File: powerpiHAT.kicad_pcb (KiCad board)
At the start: 2 copper layers, 65 x 30 mm, 36 parts, among them J1 Conn_01x10, J2 AudioJack2_Dual_Ground_Switche, J3 40HAT, J4 AudioJack2_Dual_Ground_Switche, J5 AudioJack2_Dual_Ground_Switche, J6 AudioJack2_Dual_Ground_Switche, J9 CONN_01X02, Q1 DMG2305UX, Q2 DMMT5401, U2 CAT24C32

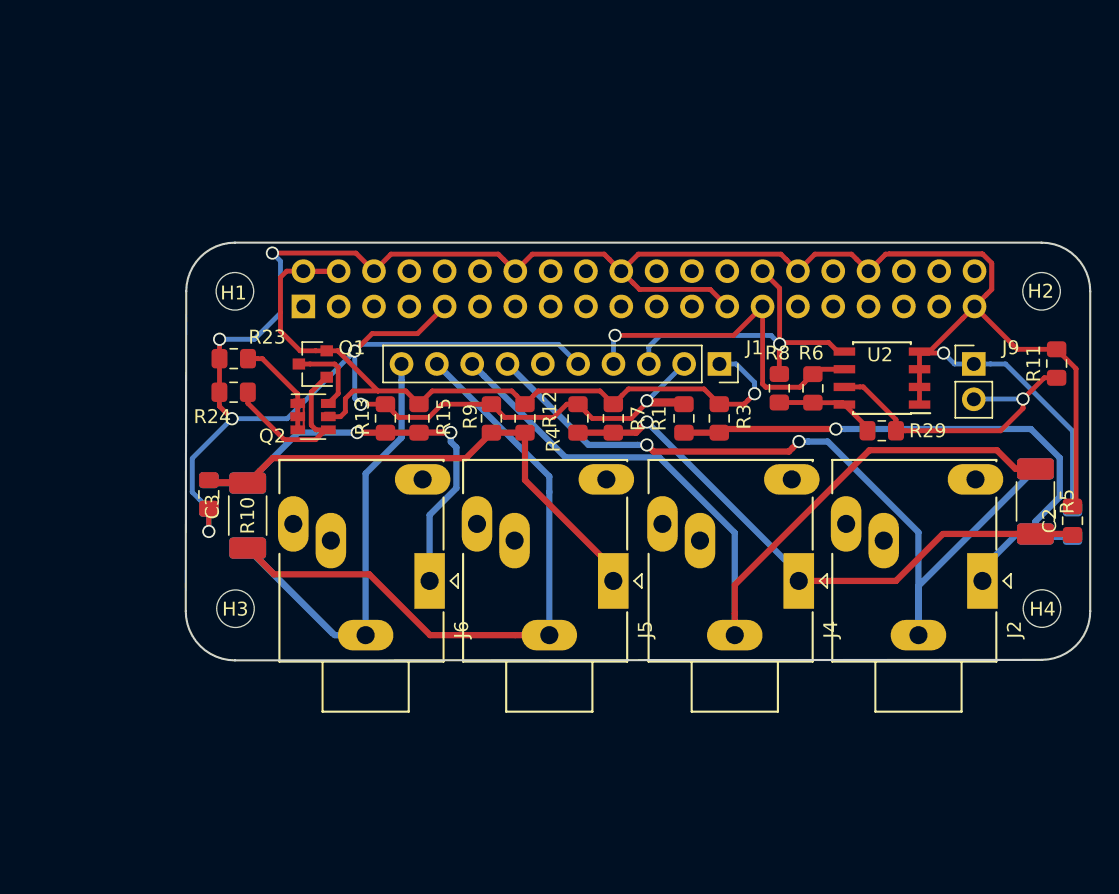
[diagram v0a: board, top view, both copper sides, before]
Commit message: Essentially, release 1.0.0 of the PowerPiHAT... we'll see if there's electrical changes necessary once we get a couple boards etched and populated.
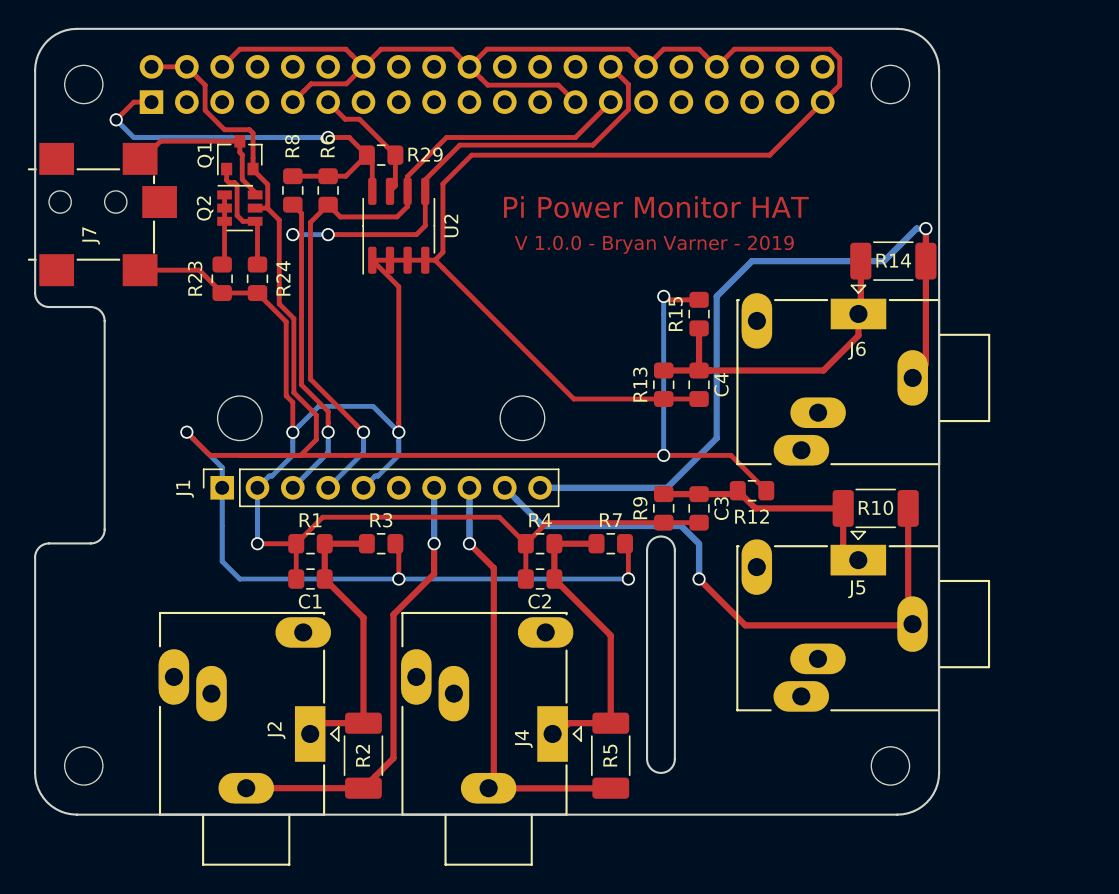
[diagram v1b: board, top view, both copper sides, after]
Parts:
- removed J9: CONN_01X02, Connector_PinHeader_2.54mm:PinHeader_1x02_P2.54mm_Vertical
- removed R11: DNP, Resistor_SMD:R_0805_2012Metric_Pad1.15x1.40mm_HandSolder
- added H5: 3mm_Mounting_Hole, MountingHole:MountingHole_3.2mm_M3_DIN965, F.Cu at (112.7, 88.0)
- added H6: 3mm_Mounting_Hole, MountingHole:MountingHole_3.2mm_M3_DIN965, F.Cu at (133.0, 88.0)
- added J7: Barrel_Jack, project_footprints:BarrellJack-DC-902_SMT_Horizontal, F.Cu at (97.3, 70.3)
- C1, C4, R14, R2: moved to F.Cu
- U2: footprint Package_SOIC:SOIC-8_3.9x4.9mm_P1.27mm -> Package_SO:SOIC-8_3.9x4.9mm_P1.27mm
- moved H4 69.8 mm to (101.5, 113.0)
- moved C1 54.9 mm to (117.8, 99.6), turned to 180 degrees
- moved R2 51.7 mm to (121.6, 112.3), turned to 90 degrees
- moved R14 49.9 mm to (159.7, 76.7), turned to 180 degrees
- moved J2 49.6 mm to (117.8, 110.7)
- moved H3 48.4 mm to (159.5, 113.0)
- moved R10 45.2 mm to (158.4, 94.5), turned to 180 degrees
- moved R29 41.1 mm to (122.9, 69.1)
- moved C2 38.5 mm to (134.3, 99.6), turned to 180 degrees
- moved R8 37.8 mm to (116.5, 71.6), turned to 270 degrees
- moved R6 37.6 mm to (119.1, 71.6), turned to 270 degrees
- moved J1 36.8 mm to (111.5, 93.0), turned to 90 degrees
- moved U2 36.4 mm to (124.2, 74.2), turned to 90 degrees
- moved J6 36.3 mm to (157.2, 80.5), turned to 180 degrees
- moved C4 36.1 mm to (145.7, 85.6)
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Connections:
- J3 pad 1: (no net) -> /P3V3_HAT
- J3 pad 11: (no net) -> /WP_EEPROM
- R29 pad 1: /P3V3 -> /P3V3_HAT
- R29 pad 2: Net-(J9-Pad2) -> /WP_EEPROM
- R6 pad 1: /P3V3 -> /P3V3_HAT
- R8 pad 1: /P3V3 -> /P3V3_HAT
- U2 pad 7: Net-(J9-Pad2) -> /WP_EEPROM
- U2 pad 8: /P3V3 -> /P3V3_HAT
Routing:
- net /P5V_HAT: track 59.3 -> 144.0 mm, vias 1 -> 5
- net /ID_SC_EEPROM: track 24.1 -> 55.9 mm, vias 1 -> 3
- net /P3V3_HAT: track 0.00 -> 30.9 mm, vias 0 -> 2
- net /ADS_A1: track 61.1 -> 30.8 mm, vias 0 -> 1
- net /ADS_A0: track 58.1 -> 32.1 mm, vias 2 -> 1
- net /ID_SD_EEPROM: track 26.1 -> 48.9 mm
- net Net-(C3-Pad1): track 40.5 -> 17.8 mm
- net GND: track 249.3 -> 226.6 mm, vias 8 -> 3
- net Net-(J9-Pad2): track 22.6 -> 0.00 mm, vias 1 -> 0
- net Net-(C1-Pad1): track 42.7 -> 21.2 mm, vias 1 -> 0
- net Net-(C2-Pad1): track 42.3 -> 21.7 mm, vias 1 -> 0
- net Net-(C4-Pad1): track 34.4 -> 23.5 mm, vias 2 -> 0
- net /ADS_A3: track 43.0 -> 52.6 mm, vias 0 -> 1
- net /WP_EEPROM: track 0.00 -> 9.18 mm
- net /P3V3: track 7.31 -> 0.00 mm
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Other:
- board size 65 x 30 mm -> 65 x 56.5 mm
- board text added: "Pi Power Monitor HAT"
- board text added: "V 1.0.0 - Bryan Varner - 2019"
